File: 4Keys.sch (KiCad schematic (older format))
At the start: 29 parts, among them J1 OLED1, J2 OLED2, SW1 SW_Reset, U1 ATmega32U4-AU, Y1 16MHz

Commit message: Hotswap
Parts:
- MXDn1, MXLeft1, MXRight1, MXUp1: footprint MX_Alps_Hybrid:MX-1U-NoLED -> MX_Only:MXOnly-1U-Hotswap
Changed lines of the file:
@@
 F 0 "MXLeft1" H 4633 2323 60  0000 C CNN
 F 1 "MX-NoLED" H 4633 2249 20  0000 C CNN
-F 2 "MX_Alps_Hybrid:MX-1U-NoLED" H 3975 2075 60  0001 C CNN
+F 2 "MX_Only:MXOnly-1U-Hotswap" H 3975 2075 60  0001 C CNN
 F 3 "" H 3975 2075 60  0001 C CNN
 	1    4600 2100
@@
 F 0 "MXDn1" H 5233 2323 60  0000 C CNN
 F 1 "MX-NoLED" H 5233 2249 20  0000 C CNN
-F 2 "MX_Alps_Hybrid:MX-1U-NoLED" H 4575 2075 60  0001 C CNN
+F 2 "MX_Only:MXOnly-1U-Hotswap" H 4575 2075 60  0001 C CNN
 F 3 "" H 4575 2075 60  0001 C CNN
 	1    5200 2100
@@
 F 0 "MXRight1" H 5958 2323 60  0000 C CNN
 F 1 "MX-NoLED" H 5958 2249 20  0000 C CNN
-F 2 "MX_Alps_Hybrid:MX-1U-NoLED" H 5300 2075 60  0001 C CNN
+F 2 "MX_Only:MXOnly-1U-Hotswap" H 5300 2075 60  0001 C CNN
 F 3 "" H 5300 2075 60  0001 C CNN
 	1    5925 2100
@@
 F 0 "MXUp1" H 5233 1598 60  0000 C CNN
 F 1 "MX-NoLED" H 5233 1524 20  0000 C CNN
-F 2 "MX_Alps_Hybrid:MX-1U-NoLED" H 4575 1350 60  0001 C CNN
+F 2 "MX_Only:MXOnly-1U-Hotswap" H 4575 1350 60  0001 C CNN
 F 3 "" H 4575 1350 60  0001 C CNN
 	1    5200 1375

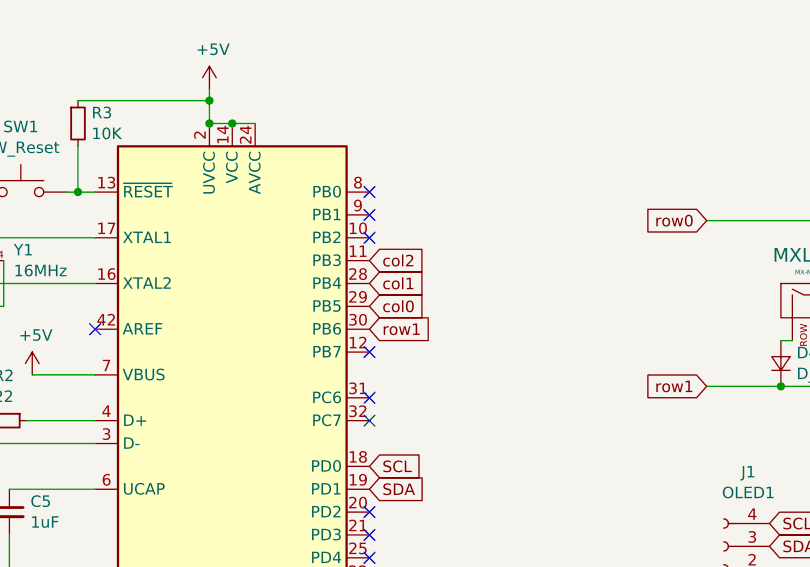
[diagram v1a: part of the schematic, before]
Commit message: Update PCB
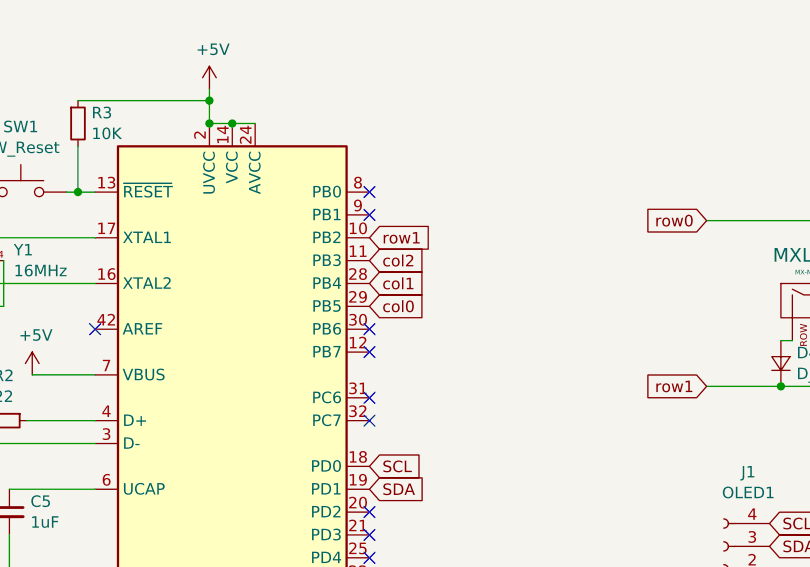
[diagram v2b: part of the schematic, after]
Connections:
- net row1: now also U1.10 (PB2); no longer U1.30 (PB6)
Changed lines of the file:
@@
 Text GLabel 2700 2000 2    50   Input ~ 0
 col1
-Text GLabel 2700 2200 2    50   Input ~ 0
+Text GLabel 2700 1800 2    50   Input ~ 0
 row1
 Text GLabel 2700 3500 2    50   Input ~ 0
@@
 NoConn ~ 2700 2500
 NoConn ~ 2700 2300
-NoConn ~ 2700 1800
 NoConn ~ 2700 1700
 NoConn ~ 2700 1600
@@
 Text GLabel 2700 1900 2    50   Input ~ 0
 col2
+NoConn ~ 2700 2200
 $EndSCHEMATC
